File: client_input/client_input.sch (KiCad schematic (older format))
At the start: 29 parts, among them P1 Analog In, P2 FTDI, P3 Ribbon, P4 Ribbon, P6 Ribbon, P7 Ribbon, P8 Ribbon, P9 LiPo, SW1 PAIR_MODE, SW2 RESET, SW3 Bootload, SW4 DIPS_08, U1 MCP3208, U2 ESP-12_Breakout, U3 MCP23017

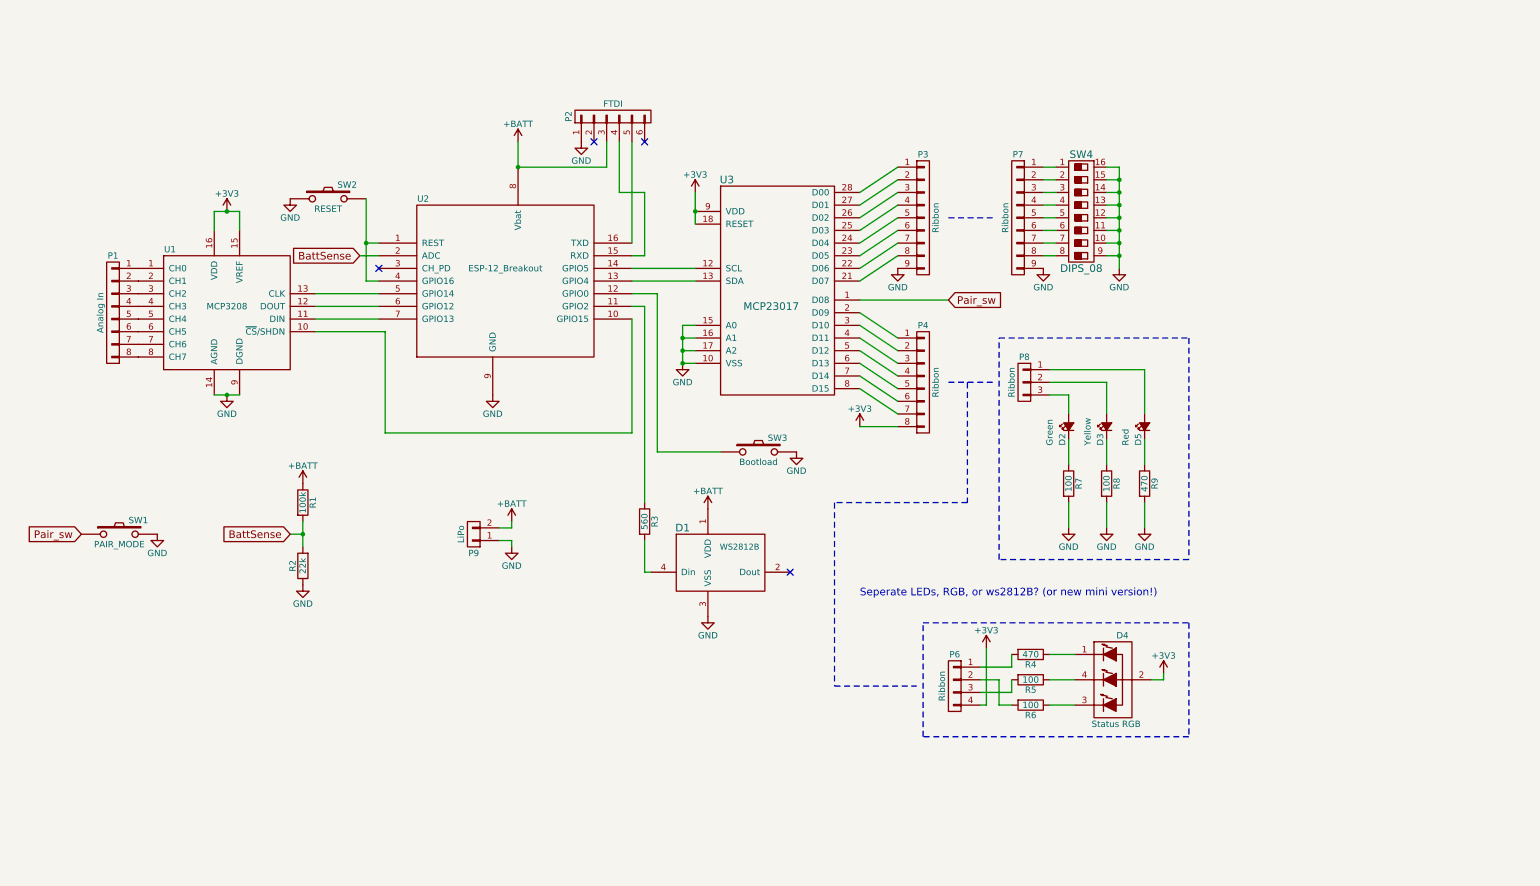
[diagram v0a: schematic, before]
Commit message: ???
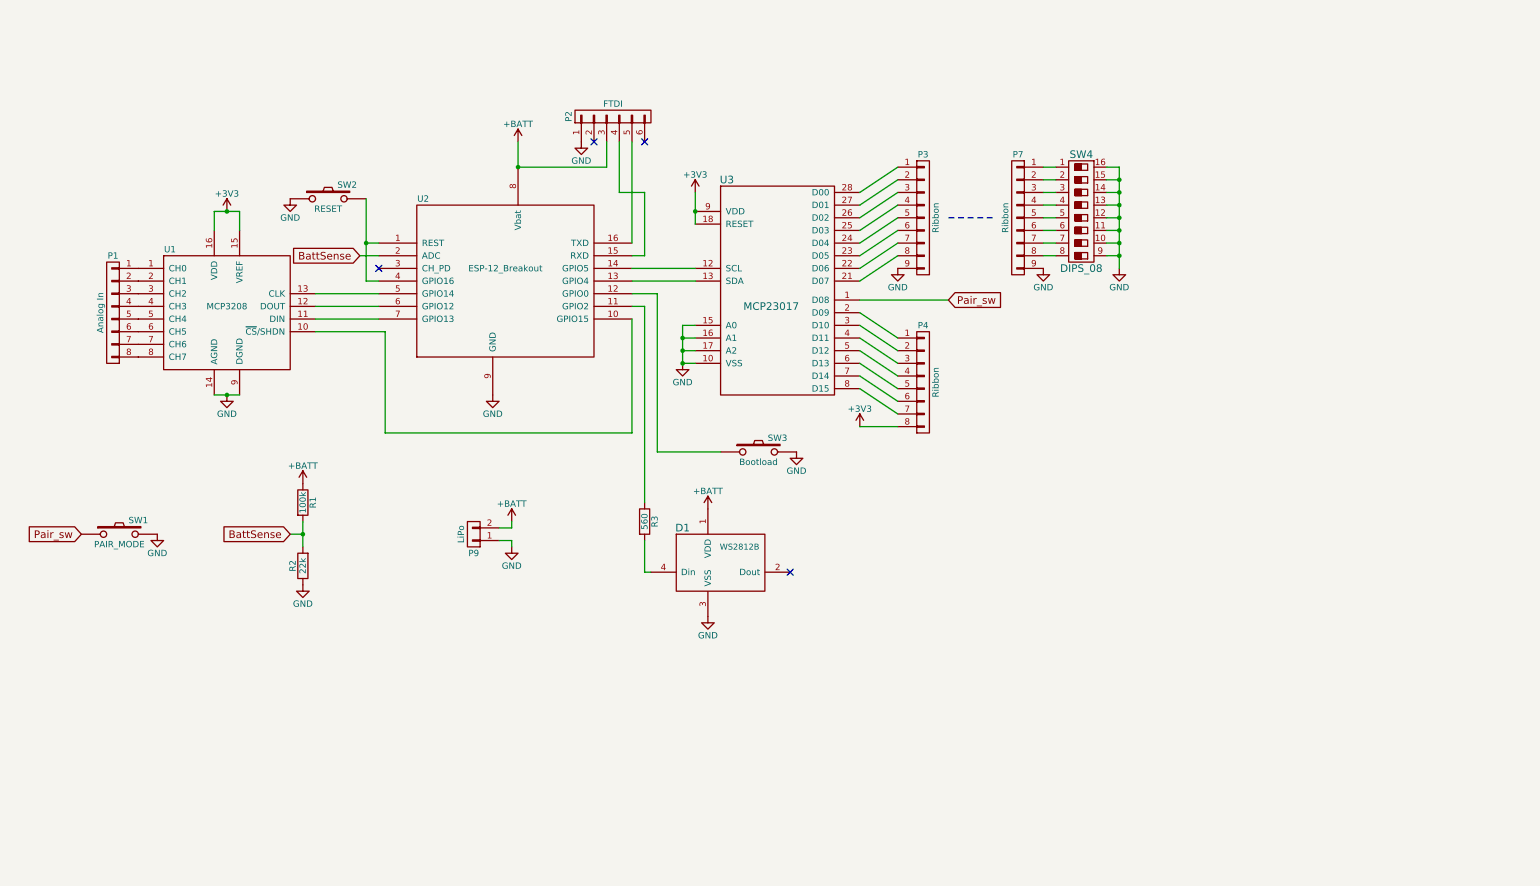
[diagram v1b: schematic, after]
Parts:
- removed D2: Green, LEDs:LED-3MM, symbol Led_Small
- removed D3: Yellow, LEDs:LED-3MM, symbol Led_Small
- removed D4: Status RGB, LEDs:LED-RGB-5MM_Common_Cathode, symbol LED_RABG
- removed D5: Red, LEDs:LED-3MM, symbol Led_Small
- removed P6: Ribbon, Socket_Strips:Socket_Strip_Straight_1x04, symbol CONN_01X04
- removed P8: Ribbon, Socket_Strips:Socket_Strip_Straight_1x03, symbol CONN_01X03
- removed R4, R9: 470, Discret:R4, symbol R
- removed R5, R6, R7, R8: 100, Discret:R4, symbol R
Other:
- note removed: "Seperate LEDs, RGB, or ws2812B? (or new mini version!)"

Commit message: version 2.0, lots of changes. (smd parts, 2 sided, production ready)
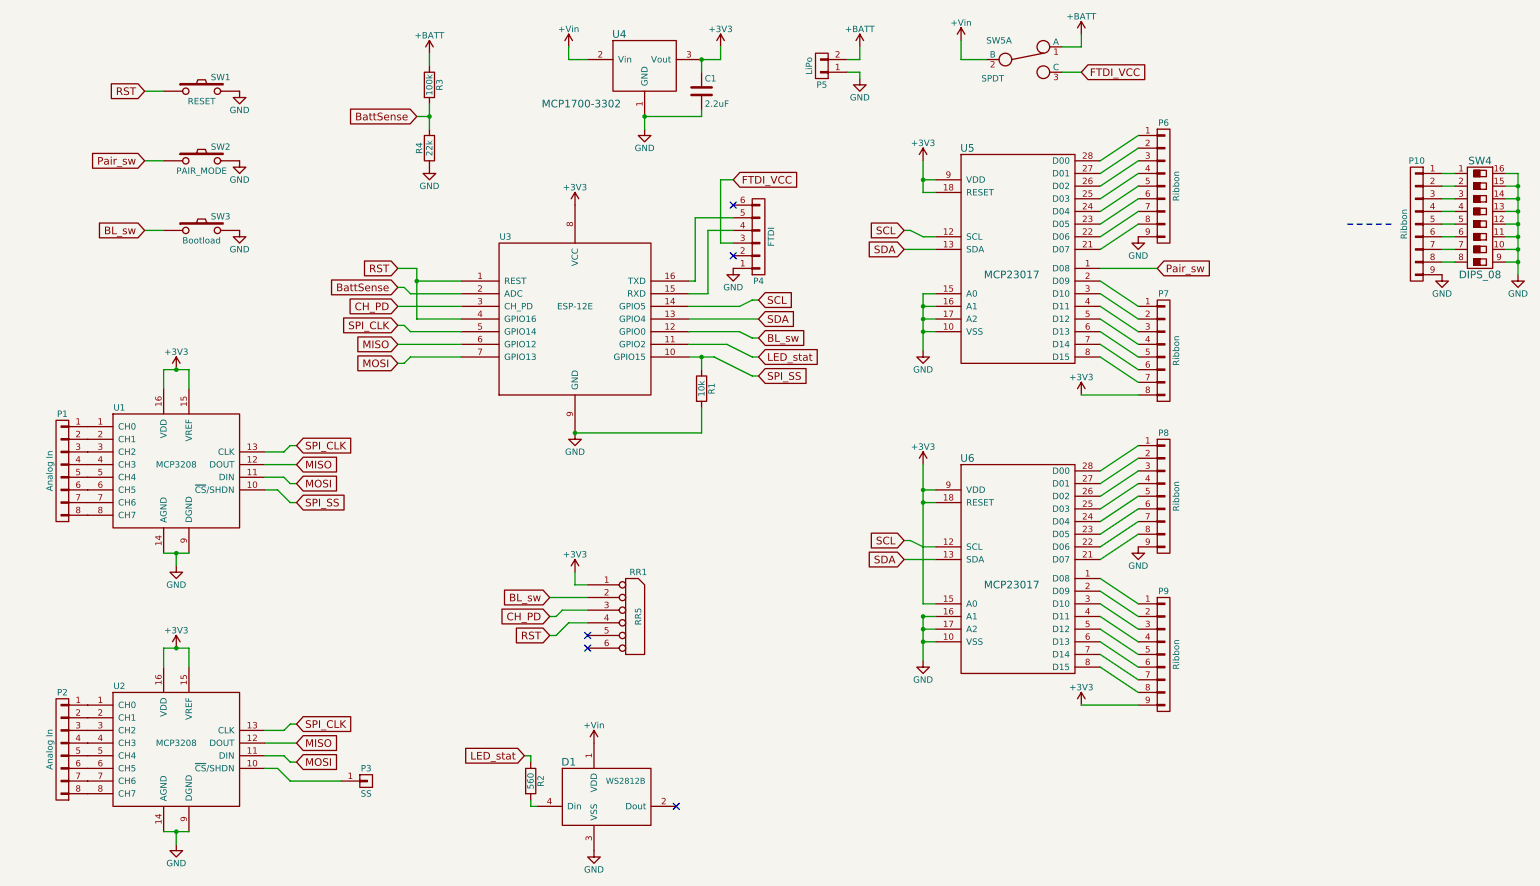
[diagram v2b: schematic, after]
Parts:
- removed U2: ESP-12_Breakout, ESP8266:ESP12_Breakout, symbol ESP-12_Breakout
- added C1: 2.2uF, Capacitors_ThroughHole:C_Disc_D3_P2.5, symbol C
- added P2: Analog In, Socket_Strips:Socket_Strip_Straight_1x08, symbol CONN_01X08
- added P3: SS, Measurement_Points:Measurement_Point_Round-TH_Small, symbol CONN_01X01
- added P8, P9: Ribbon, Socket_Strips:Socket_Strip_Straight_1x09, symbol CONN_01X09
- added R1: 10k, Discret:R4, symbol R
- added RR1: RR5, Resistors_ThroughHole:Resistor_Array_SIP5, symbol RR5
- added SW5: SPDT, Buttons_Switches_ThroughHole:SW_Micro_SPST, symbol Switch_SPDT_x2
- added U2: MCP3208, Housings_SOIC:SOIC-16_3.9x9.9mm_Pitch1.27mm, symbol MCP3008
- added U3: ESP-12E, ESP8266:ESP-12E_Brendan, symbol ESP-12
- added U4: MCP1700-3302, TO_SOT_Packages_SMD:SOT89-3_Housing_Handsoldering, symbol MCP1700-3302
- added U6: MCP23017, Housings_SOIC:SOIC-28_7.5x17.9mm_Pitch1.27mm, symbol MCP23017
- SW2: renamed from SW1; footprint Buttons_Switches_ThroughHole:SW_TH_Tactile_Omron_B3F-10xx -> Buttons_Switches_ThroughHole:SW_PUSH_SMALL
- U1: footprint Housings_DIP:DIP-16_W7.62mm_LongPads -> Housings_SOIC:SOIC-16_3.9x9.9mm_Pitch1.27mm
- U5: renamed from U3; footprint Housings_DIP:DIP-28_W7.62mm_LongPads -> Housings_SOIC:SOIC-28_7.5x17.9mm_Pitch1.27mm
- renumbered P7 to P10, P2 to P4, P9 to P5, P3 to P6, P4 to P7, R3 to R2, R1 to R3, R2 to R4, SW2 to SW1
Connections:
- net +3V3: now also C1.1, P9.9 (P9), RR1.1 (COM), U2.15 (VREF), U2.16 (VDD), U3.8 (VCC), U4.3 (Vout), U6.15 (A0), U6.18 (RESET), U6.9 (VDD)
- net +BATT: now also SW5.1 (A); no longer D1.1 (VDD), P4.3 (P3)
- net BattSense: now also U3.2 (ADC)
- net GND: now also SW1.2, C1.2, P8.9 (P9), R1.2, U2.14 (AGND), U2.9 (DGND), U3.9 (GND), U4.1 (GND), U6.10 (VSS), U6.16 (A1), U6.17 (A2); no longer SW1.1
- net SPI_SS: now reaches U1.10 (~CS~/SHDN)
- net SPI_SS: now also R1.1, U3.10 (GPIO15)
- net MOSI: now reaches U1.11 (DIN)
- net MOSI: now also U2.11 (DIN), U3.7 (GPIO13)
- net MISO: now reaches U1.12 (DOUT)
- net MISO: now also U2.12 (DOUT), U3.6 (GPIO12)
- net SPI_CLK: now reaches U1.13 (CLK)
- net SPI_CLK: now also U2.13 (CLK), U3.5 (GPIO14)
- net LED_stat: now reaches R2.1
- net LED_stat: now also U3.11 (GPIO2)
- net BL_sw: now reaches SW3.1
- net BL_sw: now also RR1.2, U3.12 (GPIO0)
- net SDA: now reaches U5.13 (SDA)
- net SDA: now also U3.13 (GPIO4), U6.13 (SDA)
- net SCL: now reaches U5.12 (SCL)
- net SCL: now also U3.14 (GPIO5), U6.12 (SCL)
- net at P4.4 (P4): now also U3.15 (RXD)
- net at P4.5 (P5): now also U3.16 (TXD)
- new net: P9.1 (P1), U6.1 (D08)
- new net: P9.2 (P2), U6.2 (D09)
- new net: P8.8 (P8), U6.21 (D07)
- new net: P8.7 (P7), U6.22 (D06)
- new net: P8.6 (P6), U6.23 (D05)
- new net: P8.5 (P5), U6.24 (D04)
- new net: P8.4 (P4), U6.25 (D03)
- new net: P8.3 (P3), U6.26 (D02)
- new net: P8.2 (P2), U6.27 (D01)
- new net: P8.1 (P1), U6.28 (D00)
- new net: P9.3 (P3), U6.3 (D10)
- new net: P9.4 (P4), U6.4 (D11)
- new net: P9.5 (P5), U6.5 (D12)
- new net: P9.6 (P6), U6.6 (D13)
- new net: P9.7 (P7), U6.7 (D14)
- new net: P9.8 (P8), U6.8 (D15)
- new net: P2.1 (P1), U2.1 (CH0)
- new net: P3.1 (P1), U2.10 (~CS~/SHDN)
- new net: P2.2 (P2), U2.2 (CH1)
- new net: P2.3 (P3), U2.3 (CH2)
- new net: P2.4 (P4), U2.4 (CH3)
- new net: P2.5 (P5), U2.5 (CH4)
- new net: P2.6 (P6), U2.6 (CH5)
- new net: P2.7 (P7), U2.7 (CH6)
- new net: P2.8 (P8), U2.8 (CH7)
- new net +Vin: D1.1 (VDD), SW5.2 (B), U4.2 (Vin)
- new net CH_PD: RR1.3, U3.3 (CH_PD)
- new net FTDI_VCC: P4.3 (P3), SW5.3 (C)
- new net RST: RR1.4, SW1.1, U3.1 (REST), U3.4 (GPIO16)
- no-connect marks 4 -> 5
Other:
- moved on the sheet: D1, P1, P10, P4, P5, P6, P7, R2, R3, R4, SW1, SW2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
